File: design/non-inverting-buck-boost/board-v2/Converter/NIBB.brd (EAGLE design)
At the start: 93.9 x 39.4 mm, 8 parts

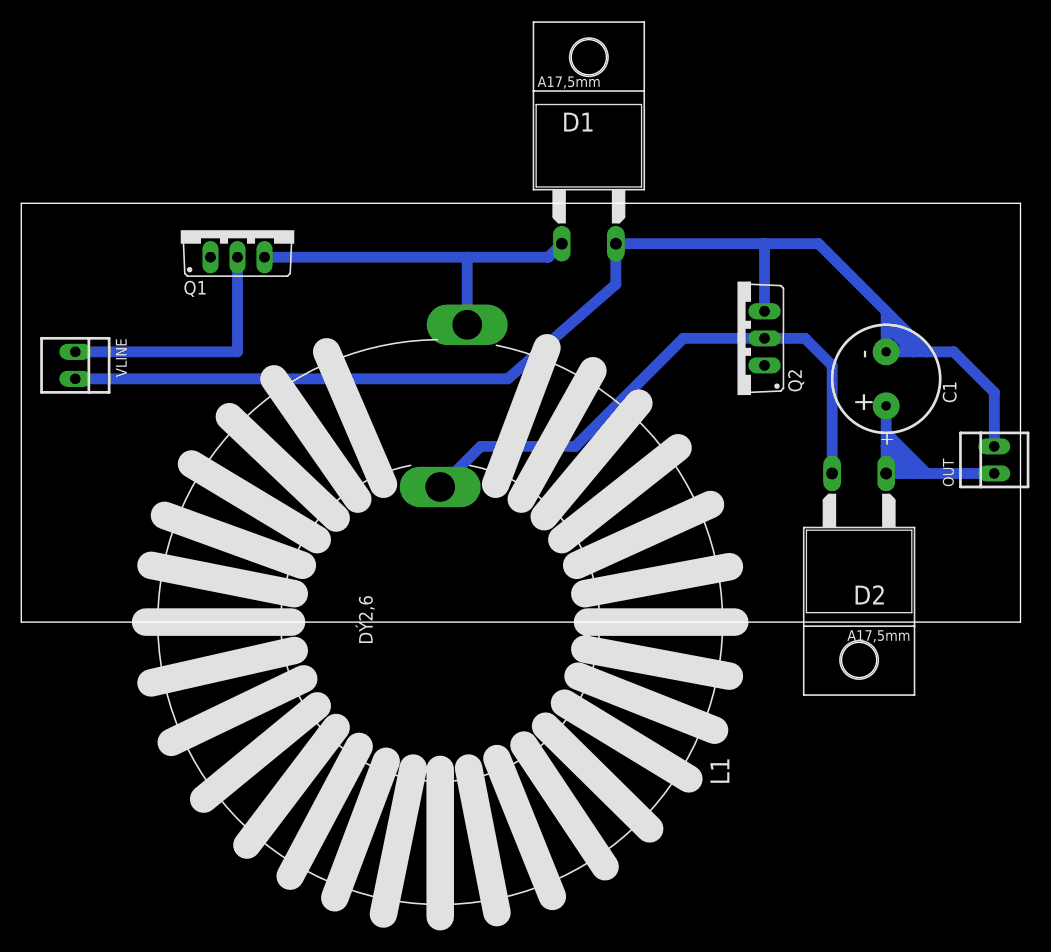
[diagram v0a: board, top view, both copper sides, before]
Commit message: finished power board layout
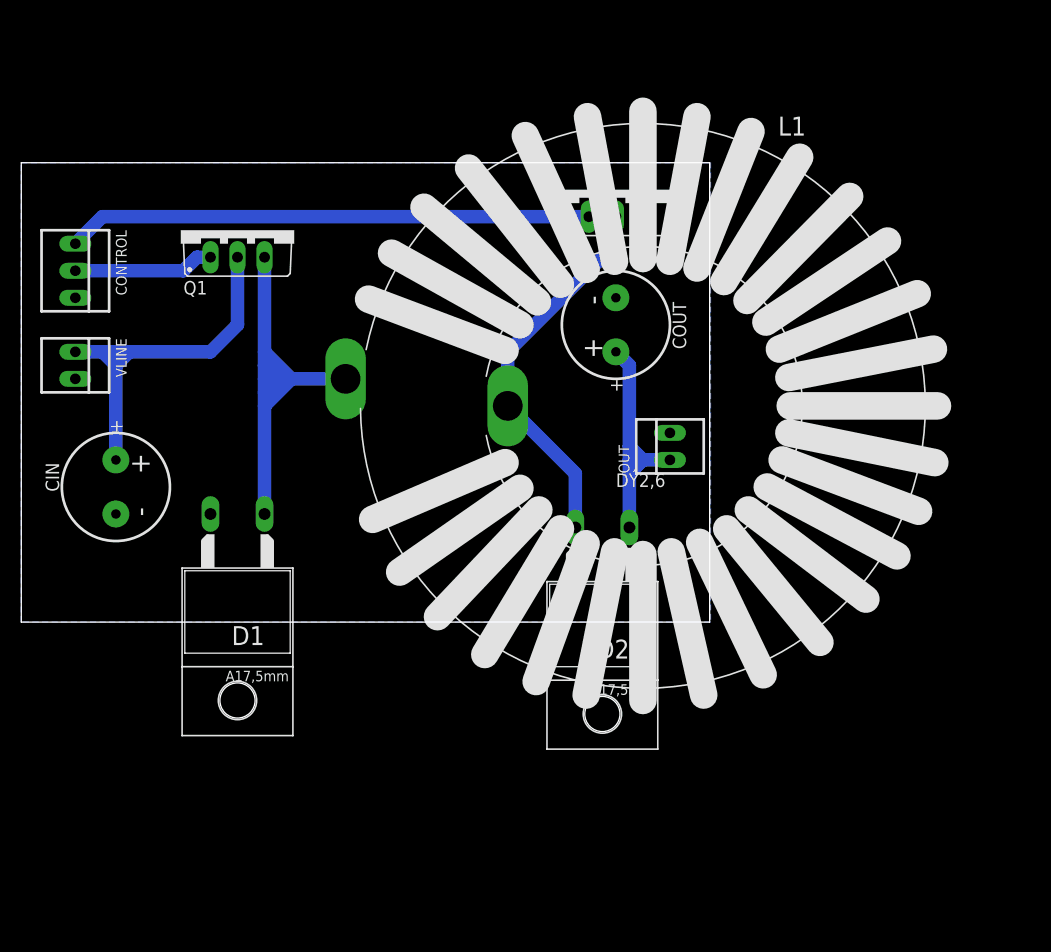
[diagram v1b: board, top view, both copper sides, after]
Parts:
- removed C1: (no value), capacitor:20ROUND40P
- added CIN, COUT: (no value), capacitor:20ROUND40P
- added CONTROL: 22-23-2031, con-molex:22-23-2031
- moved D1 50.4 mm to (20.3, 3.81), turned to 180 degrees
- moved OUT 30.5 mm to (61.0, 16.5)
- moved L1 27.9 mm to (58.4, 20.3), turned to 0 degrees
- moved D2 24.7 mm to (54.6, 2.54)
- moved Q2 18.1 mm to (55.9, 40.6), turned to 0 degrees
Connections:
- removed net N$4: C1.-, D1.A, OUT.2, Q2.S, VLINE.2
- removed net N$5: Q1.G
- new net CONTROL1: CONTROL.1, Q2.G
- new net CONTROL2: CONTROL.2, Q1.G
- new net GND: CIN.-, CONTROL.3, COUT.-, D1.A, OUT.2, Q2.S, VLINE.2
- net N$3: now also CIN.+
- net N$7: now also COUT.+; no longer C1.+
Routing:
- net N$4: track 121.9 -> 0.00 mm
- net CONTROL1: track 0.00 -> 49.3 mm
- net N$2: track 53.8 -> 36.0 mm
- net CONTROL2: track 0.00 -> 13.2 mm
- net N$3: track 24.1 -> 36.4 mm
- net N$1: track 34.8 -> 42.5 mm
- net N$7: track 27.3 -> 24.4 mm
- added copper zone on layer 16, net GND
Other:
- board size 93.9 x 39.4 mm -> 64.7 x 43.2 mm
